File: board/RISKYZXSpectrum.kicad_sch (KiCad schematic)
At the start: 26 parts, among them CN1 MSX_CART, IC8 LM1117MPX-3.3, J1 Conn_01x02, J2 Conn_01x02, J7 USB_1, J8 Conn_01x02, U1 CH32V307VCT6

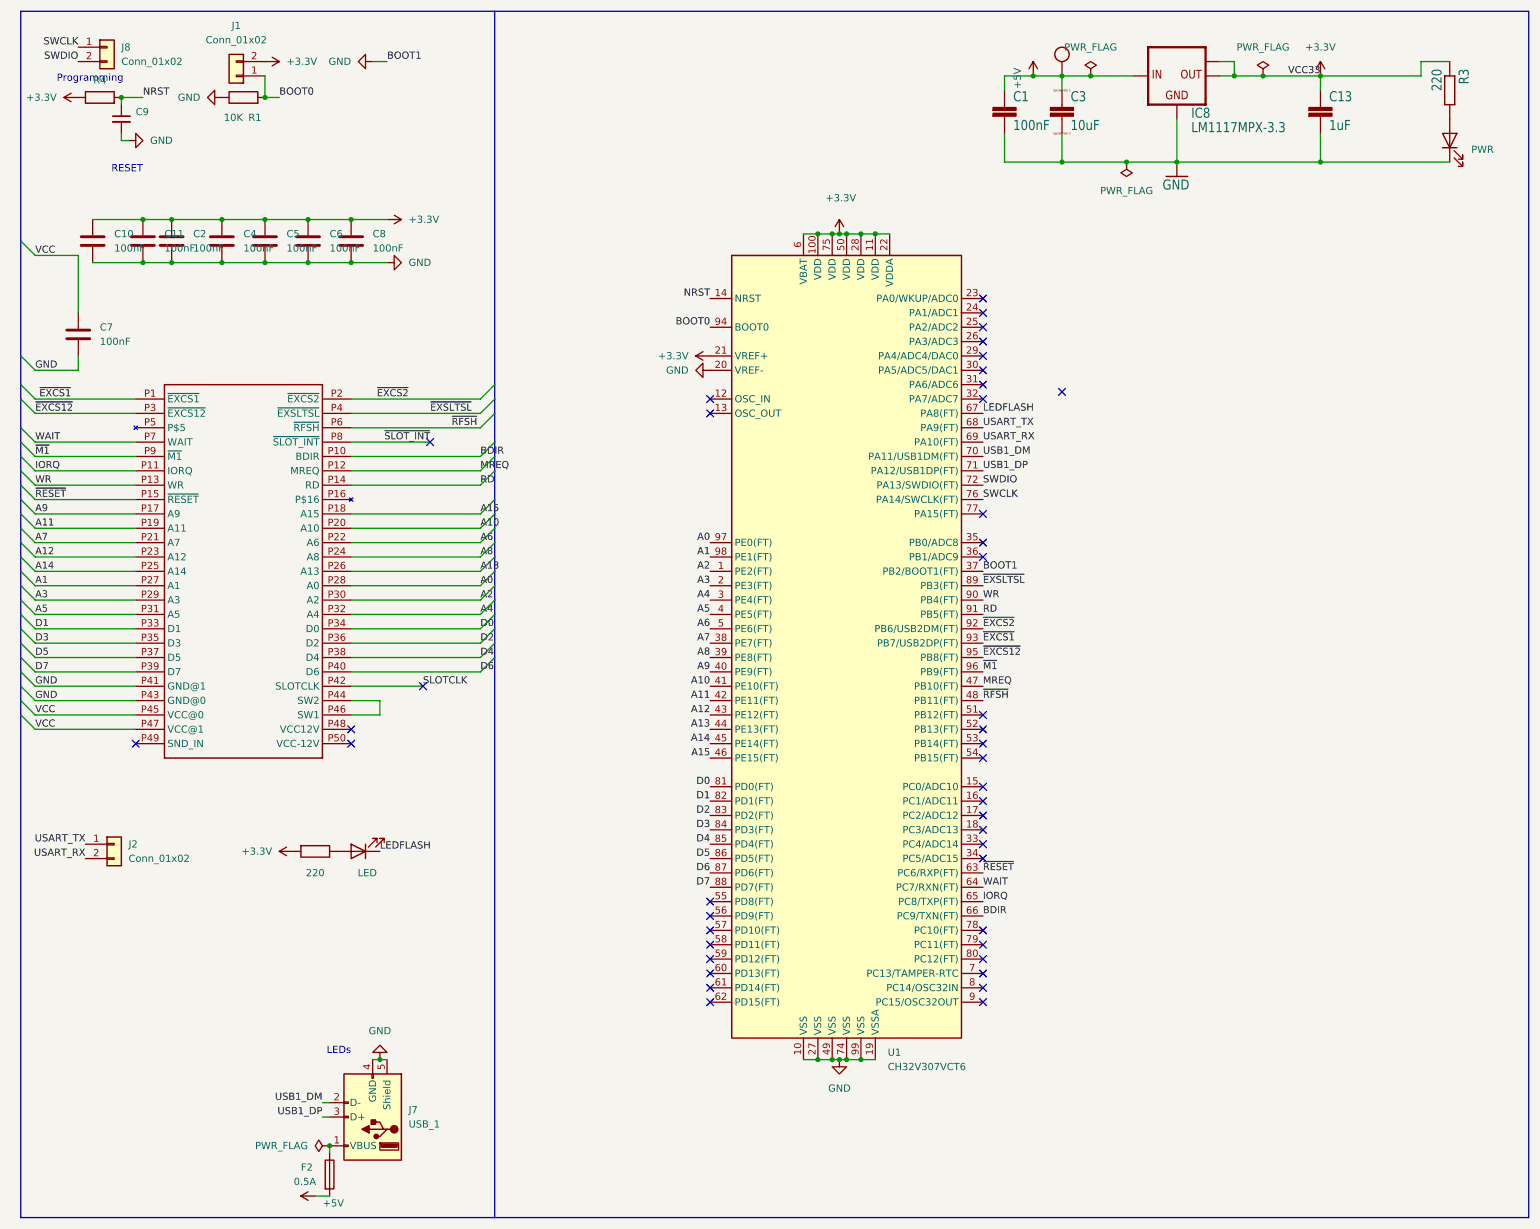
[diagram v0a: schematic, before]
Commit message: Initial PCB
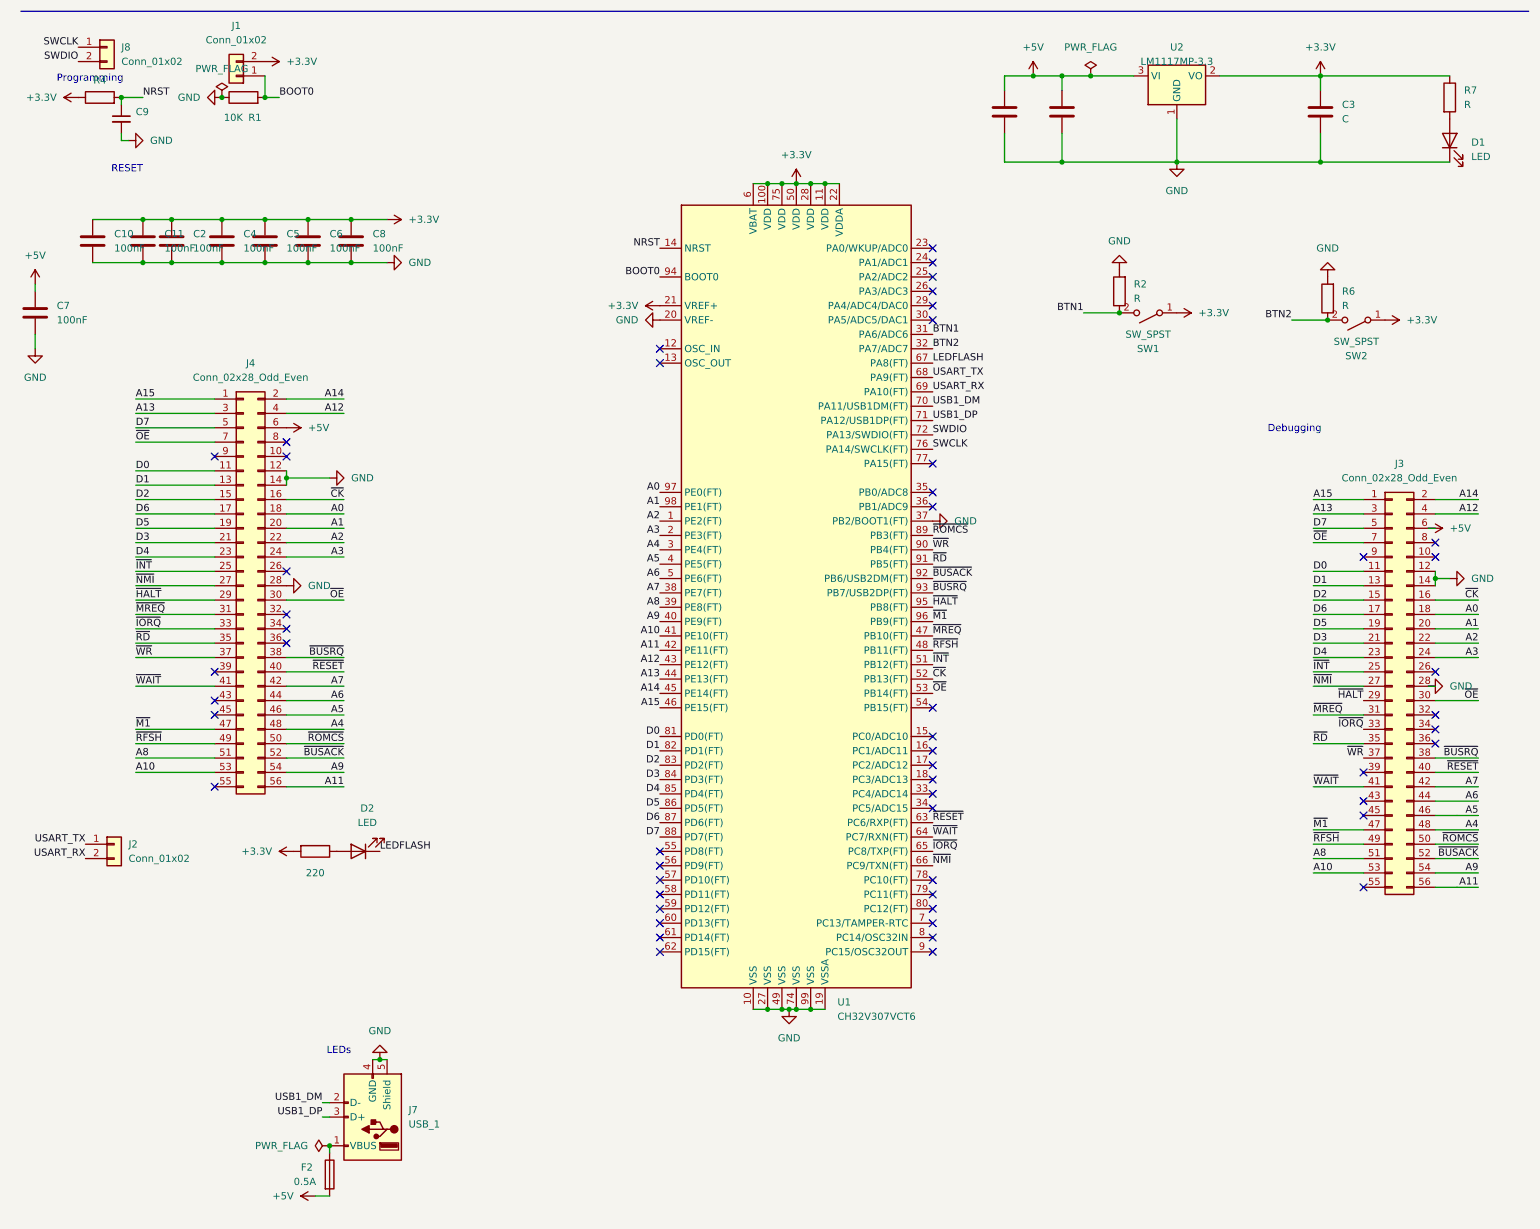
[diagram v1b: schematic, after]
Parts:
- removed C1: 100nF, tfcart:C1206, symbol tfcart-eagle-import:C-EUC1206
- removed C13: 1uF, tfcart:C1206, symbol tfcart-eagle-import:C-EUC1206
- removed C3: 10uF, tfcart:C0603, symbol tfcart-eagle-import:CC0603
- removed CN1: MSX_CART, tfcart:MSX_CART, symbol tfcart-eagle-import:MSX_CART
- removed D5: PWR, LED_SMD:LED_0805_2012Metric_Pad1.15x1.40mm_HandSolder, symbol Device:LED
- removed IC8: LM1117MPX-3.3, tfcart:SOT223, symbol tfcart-eagle-import:LM1117MPX-
- removed R3: 220, tfcart:R0603, symbol tfcart-eagle-import:R-EU_R0603
- added C1, C12, C3: C, Capacitor_SMD:C_0603_1608Metric_Pad1.08x0.95mm_HandSolder, symbol Device:C
- added D2: LED, LED_SMD:LED_0805_2012Metric_Pad1.15x1.40mm_HandSolder, symbol Device:LED
- added J3, J4: Conn_02x28_Odd_Even, Connector_PinSocket_2.54mm:PinSocket_2x28_P2.54mm_Vertical, symbol Connector_Generic:Conn_02x28_Odd_Even
- added R2, R6, R7: R, Resistor_SMD:R_0603_1608Metric_Pad0.98x0.95mm_HandSolder, symbol Device:R
- added SW1, SW2: SW_SPST, Button_Switch_THT:SW_PUSH_6mm, symbol Switch:SW_SPST
- added U2: LM1117MP-3.3, Package_TO_SOT_SMD:SOT-223-3_TabPin2, symbol Regulator_Linear:LM1117MP-3.3
- J7: footprint Connector_USB:USB_A_CONNFLY_DS1095-WNR0 -> Connector_USB:USB_A_Connfly_DS1095
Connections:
- net +3.3V: now also C3.1, R7.1, SW1.1 (A), SW2.1 (A), U2.2 (VO)
- net +5V: now also C1.1, C12.1, J3.6 (Pin_6), J4.6 (Pin_6), U2.3 (VI)
- net A0: now also J3.18 (Pin_18), J4.18 (Pin_18)
- net A1: now also J3.20 (Pin_20), J4.20 (Pin_20)
- net A10: now also J3.53 (Pin_53), J4.53 (Pin_53)
- net A11: now also J3.56 (Pin_56), J4.56 (Pin_56)
- net A12: now also J3.4 (Pin_4), J4.4 (Pin_4)
- net A13: now also J3.3 (Pin_3), J4.3 (Pin_3)
- net A14: now also J3.2 (Pin_2), J4.2 (Pin_2)
- net A15: now also J3.1 (Pin_1), J4.1 (Pin_1)
- net A2: now also J3.22 (Pin_22), J4.22 (Pin_22)
- net A3: now also J3.24 (Pin_24), J4.24 (Pin_24)
- net A4: now also J3.48 (Pin_48), J4.48 (Pin_48)
- net A5: now also J3.46 (Pin_46), J4.46 (Pin_46)
- net A6: now also J3.44 (Pin_44), J4.44 (Pin_44)
- net A7: now also J3.42 (Pin_42), J4.42 (Pin_42)
- net A8: now also J3.51 (Pin_51), J4.51 (Pin_51)
- net A9: now also J3.54 (Pin_54), J4.54 (Pin_54)
- net D0: now also J3.11 (Pin_11), J4.11 (Pin_11)
- net D1: now also J3.13 (Pin_13), J4.13 (Pin_13)
- net D2: now also J3.15 (Pin_15), J4.15 (Pin_15)
- net D3: now also J3.21 (Pin_21), J4.21 (Pin_21)
- net D4: now also J3.23 (Pin_23), J4.23 (Pin_23)
- net D5: now also J3.19 (Pin_19), J4.19 (Pin_19)
- net D6: now also J3.17 (Pin_17), J4.17 (Pin_17)
- net D7: now also J3.5 (Pin_5), J4.5 (Pin_5)
- net GND: now also D1.1 (K), C1.2, C12.2, C3.2, J3.12 (Pin_12), J3.14 (Pin_14), J3.28 (Pin_28), J4.12 (Pin_12), J4.14 (Pin_14), J4.28 (Pin_28), R2.2, R6.2, U2.1 (GND)
- net LEDFLASH: now also D2.1 (K); no longer D1.1 (K)
- net ~{M1}: now also J3.47 (Pin_47), J4.47 (Pin_47)
- net ~{RESET}: now also J3.40 (Pin_40), J4.40 (Pin_40)
- net ~{RFSH}: now also J3.49 (Pin_49), J4.49 (Pin_49)
- net at R5.1: now also D2.2 (A); no longer D1.2 (A)
- net BTN1: now reaches U1.31 (PA6/ADC6)
- net BTN1: now also R2.1, SW1.2 (B)
- net BTN2: now reaches U1.32 (PA7/ADC7)
- net BTN2: now also R6.1, SW2.2 (B)
- net ~{INT}: now reaches U1.51 (PB12(FT))
- net ~{INT}: now also J3.25 (Pin_25), J4.25 (Pin_25)
- net ~{CK}: now reaches U1.52 (PB13(FT))
- net ~{CK}: now also J3.16 (Pin_16), J4.16 (Pin_16)
- net ~{OE}: now reaches U1.53 (PB14(FT))
- net ~{OE}: now also J3.30 (Pin_30), J3.7 (Pin_7), J4.30 (Pin_30), J4.7 (Pin_7)
- net BDIR renamed ~{NMI}
- net ~{NMI}: now also J3.27 (Pin_27), J4.27 (Pin_27)
- net IORQ renamed ~{IORQ}
- net ~{IORQ}: now also J3.33 (Pin_33), J4.33 (Pin_33)
- net MREQ renamed ~{MREQ}
- net ~{MREQ}: now also J3.31 (Pin_31), J4.31 (Pin_31)
- net RD renamed ~{RD}
- net ~{RD}: now also J3.35 (Pin_35), J4.35 (Pin_35)
- net WAIT renamed ~{WAIT}
- net ~{WAIT}: now also J3.41 (Pin_41), J4.41 (Pin_41)
- net WR renamed ~{WR}
- net ~{WR}: now also J3.37 (Pin_37), J4.37 (Pin_37)
- net ~{EXCS12} renamed ~{HALT}
- net ~{HALT}: now also J3.29 (Pin_29), J4.29 (Pin_29)
- net ~{EXCS1} renamed ~{BUSRQ}
- net ~{BUSRQ}: now also J3.38 (Pin_38), J4.38 (Pin_38)
- net ~{EXCS2} renamed ~{BUSACK}
- net ~{BUSACK}: now also J3.52 (Pin_52), J4.52 (Pin_52)
- net ~{EXSLTSL} renamed ~{ROMCS}
- net ~{ROMCS}: now also J3.50 (Pin_50), J4.50 (Pin_50)
- new net: D1.2 (A), R7.2
- no-connect marks 43 -> 54
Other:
- note added: "Debugging"
- moved on the sheet: C7, U1
